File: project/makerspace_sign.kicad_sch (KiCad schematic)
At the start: 24 parts, among them J1 Conn_EXT, J2 Conn_E1_M, J3 Conn_E1_F, J4 Conn_OTH_M, J5 Conn_OTH_F, J6 Conn_E2_F, J7 Conn_E2_M

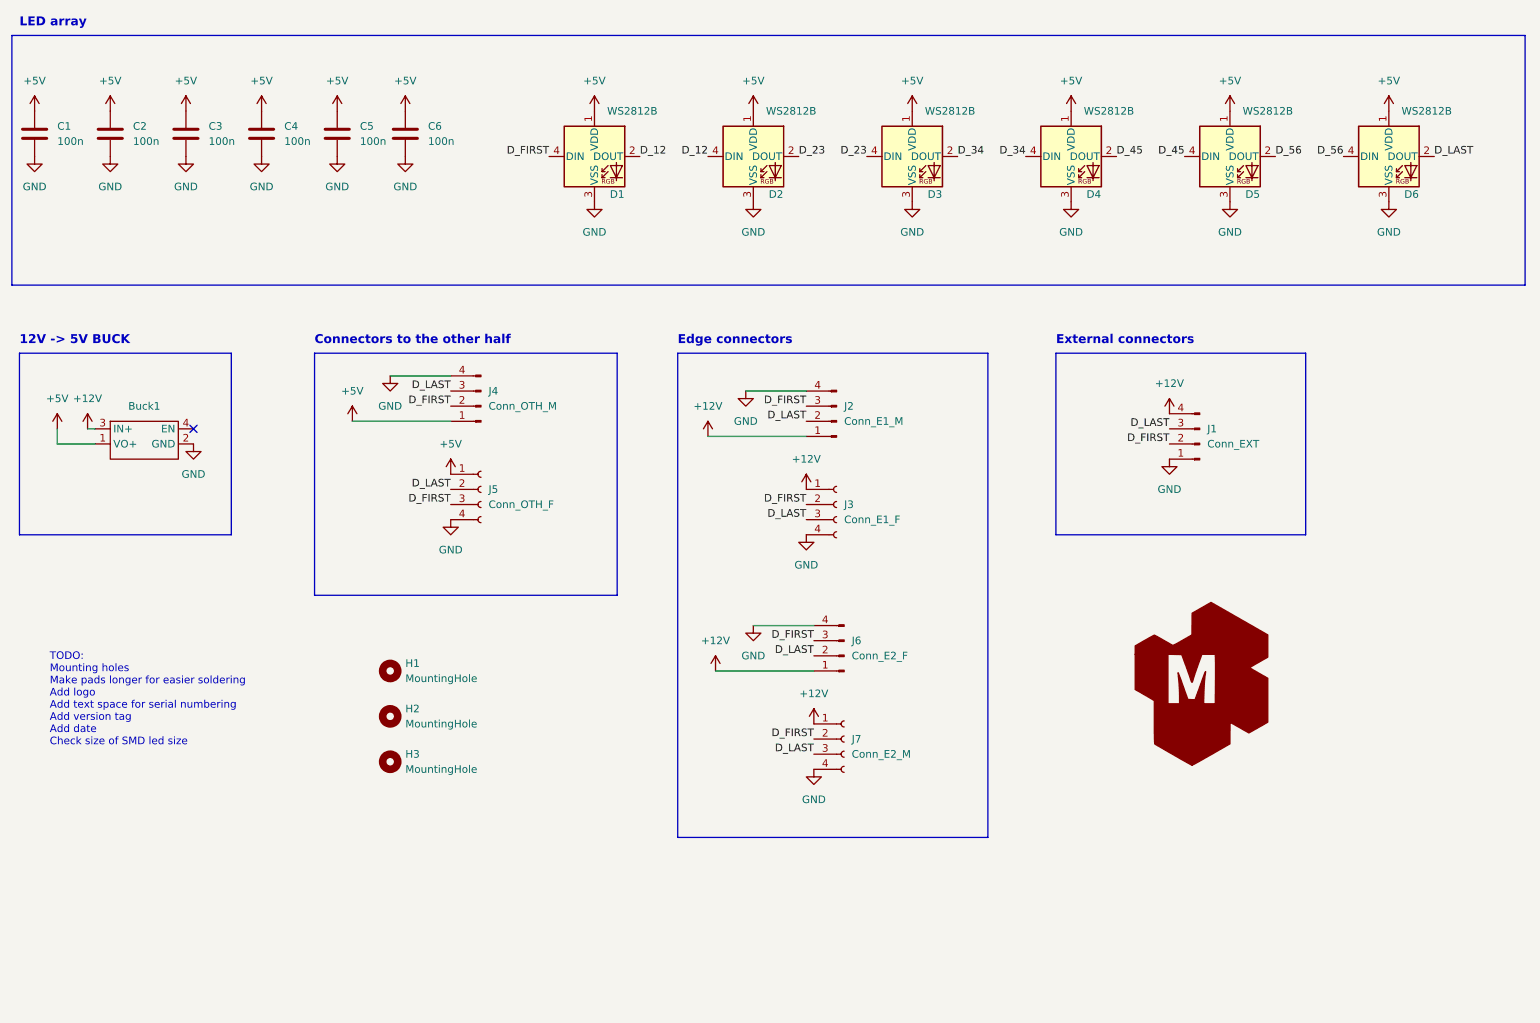
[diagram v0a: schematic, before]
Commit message: 2.1
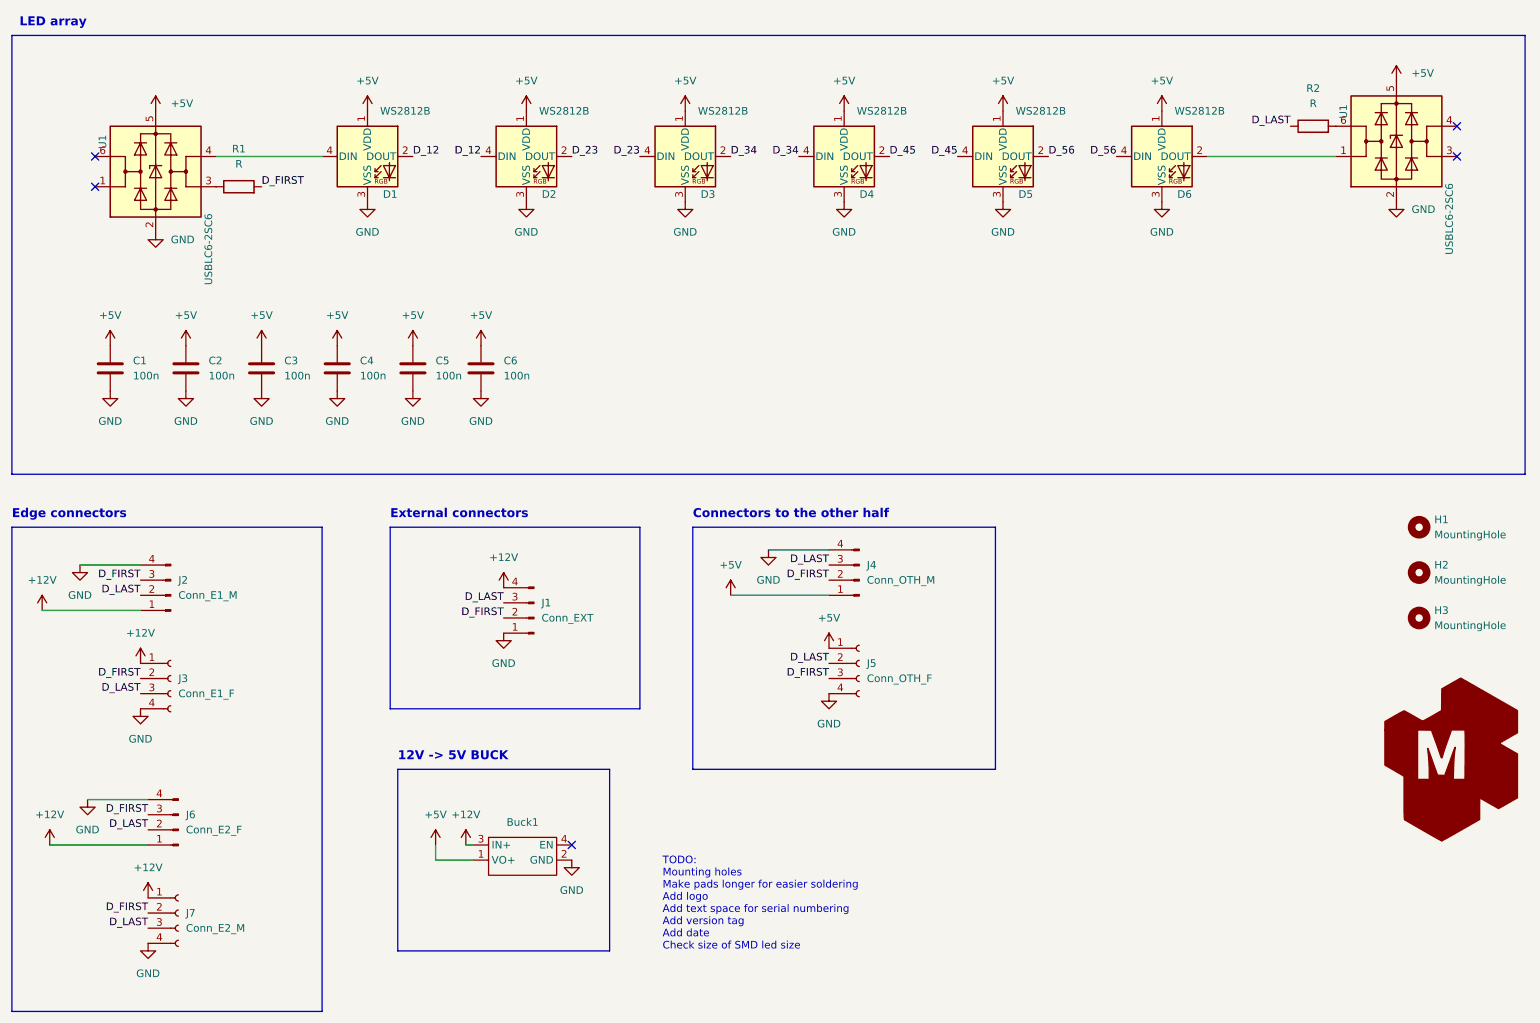
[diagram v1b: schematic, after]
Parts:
- added R1, R2: R, Resistor_SMD:R_0805_2012Metric_Pad1.20x1.40mm_HandSolder, symbol Device:R
- added U1 (x2): USBLC6-2SC6, Package_TO_SOT_SMD:SOT-23-6, symbol Power_Protection:USBLC6-2SC6
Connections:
- net +5V: now also U1.5 (VBUS), U1.5 (VBUS)
- net D_FIRST: now also R1.2; no longer D1.4 (DIN)
- net D_LAST: now also R2.1; no longer D6.2 (DOUT)
- net GND: now also U1.2 (GND), U1.2 (GND)
- new net: R1.1, U1.3 (I/O2)
- new net: D1.4 (DIN), U1.4 (I/O2)
- new net: R2.2, U1.6 (I/O1)
- new net: D6.2 (DOUT), U1.1 (I/O1)
- no-connect marks 1 -> 5
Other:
- moved on the sheet: Buck1, C1, C2, C3, C4, C5, C6, D1, D2, D3, D4, D5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
